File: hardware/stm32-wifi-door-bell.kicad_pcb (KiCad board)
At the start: 2 copper layers, 94 parts, among them J101 USB, M101 Mounting Hole, M102 Mounting Hole, M103 Mounting Hole, M104 Mounting Hole, P101 SWD, P102 FTDI-PLUG, P201 FRONT, P202 BACK, P401 P03, P601 SPEAKER, U101 STM32F072CBT6, U201 OPAMP-DUAL, U202 OPAMP-DUAL, U203 OPAMP-DUAL, U301 MC34063A, U401 TICC3000, U501 MICROSD-AMPHENOL-114-00841-68, U601 LM1875, X101 32.768kHz, X102 8MHz, X401 2500AT44M0400E

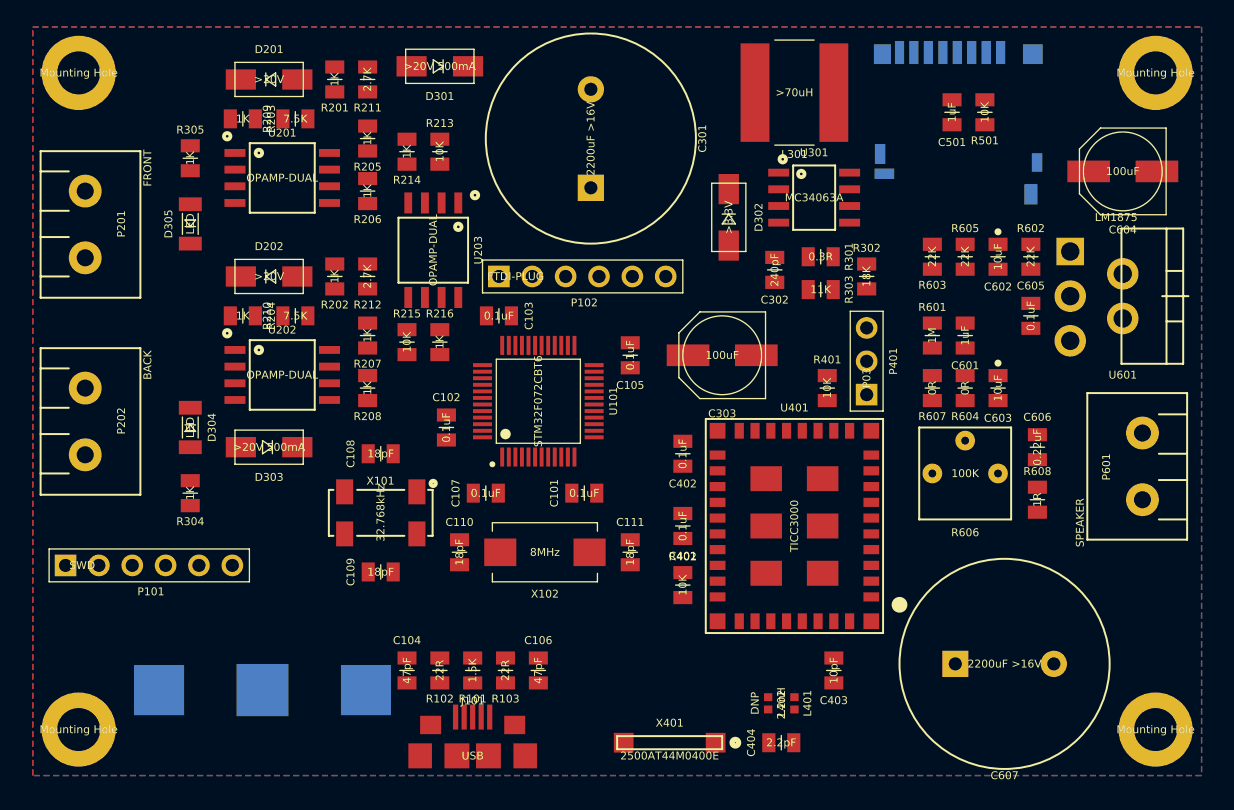
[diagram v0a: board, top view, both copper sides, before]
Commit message: clean up pcb
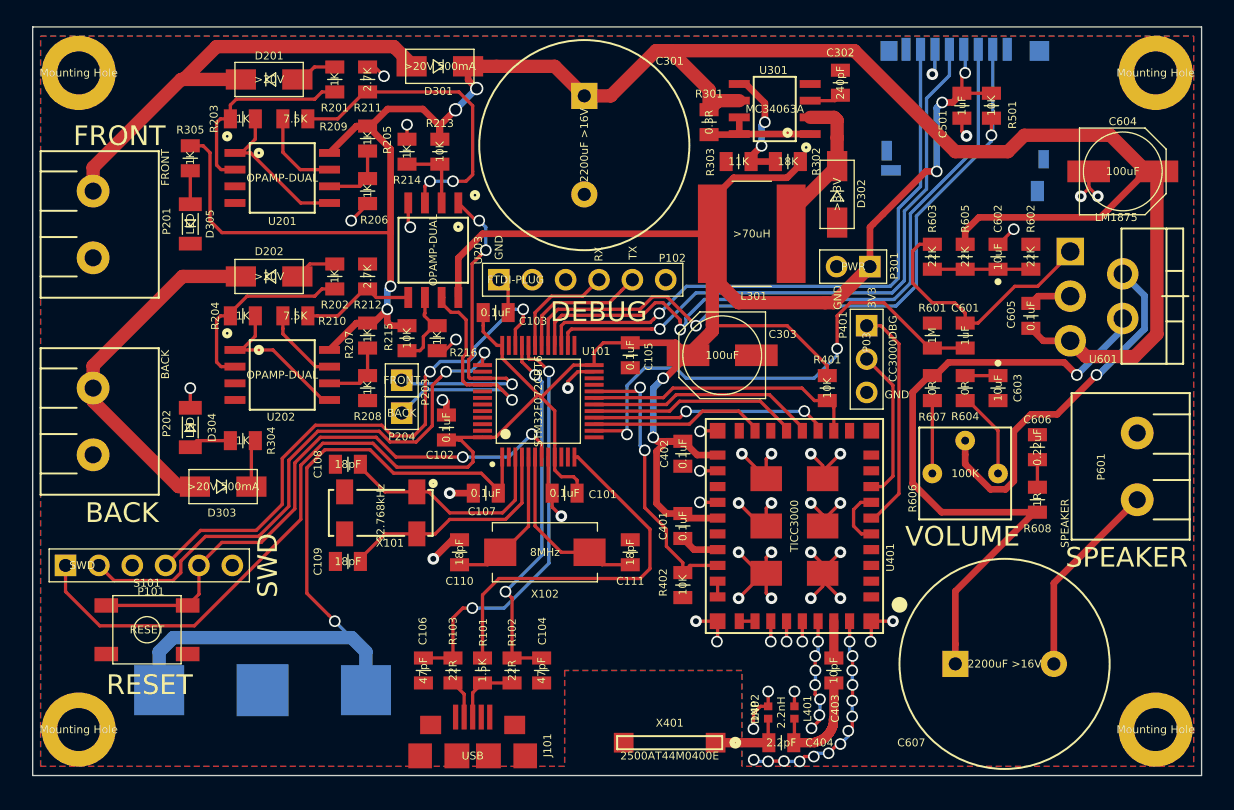
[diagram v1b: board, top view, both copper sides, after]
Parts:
- added P203: FRONT, kicadlib:HDRV1W66P254_1X1_254X249X838P, F.Cu at (88.1, 78.4)
- added P204: BACK, kicadlib:HDRV1W66P254_1X1_254X249X838P, F.Cu at (88.1, 80.9)
- added P301: PWR, kicadlib:HDRV2W66P254_1X2_508X249X838P, F.Cu at (123.8, 69.8)
- added S101: RESET, kicadlib:CKCOMP-PTS525SM10SMTR, F.Cu at (68.7, 97.4)
- P201, P202, P601: footprint kicadlib:OST-OSTTC022162 -> kicadlib:OST-OSTTA024163
- moved C302 15.1 mm to (121.5, 55.8), turned to 90 degrees
- moved R301 13.3 mm to (111.5, 58.8), turned to 270 degrees
- moved R303 11.6 mm to (113.8, 61.8)
- moved L301 11.2 mm to (114.8, 67.2), turned to 180 degrees
- moved R302 10.6 mm to (117.5, 61.8), turned to 0 degrees
- moved C104 10.2 mm to (98.8, 100.5)
- moved C106 8.75 mm to (89.8, 100.5)
- moved D302 8.43 mm to (121.2, 64.2)
- moved U301 7.39 mm to (116.5, 57.8), turned to 180 degrees
- moved R304 5.66 mm to (76.0, 83.0), turned to 0 degrees
- moved R102 5.50 mm to (96.5, 100.5)
- moved P401 5.25 mm to (123.5, 74.2), turned to 270 degrees
- moved D303 4.61 mm to (74.5, 86.5)
- moved R103 4.00 mm to (92.0, 100.5)
- moved C108 2.62 mm to (84.0, 84.8)
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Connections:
- net Net-(C403-Pad1) renamed /wifi/ANT-NET-0
- net Net-(C403-Pad2) renamed /wifi/ANT-NET-1
- net Net-(C404-Pad2) renamed /wifi/ANT-NET-2
- U101 pad 12: Net-(U101-Pad12) -> /USBDPPU
- U101 pad 18: /wifi/CS -> /wifi/IRQ
- U101 pad 19: /wifi/IRQ -> /wifi/CS
- U101 pad 38: /USBDPPU -> Net-(U101-Pad38)
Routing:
- net +3.3V: track 0.00 -> 206.4 mm, vias 0 -> 5
- net Vcc: track 0.00 -> 170.6 mm, vias 0 -> 4
- net GNDPWR: track 0.00 -> 125.1 mm, vias 0 -> 66
- net Net-(BT101-Pad1): track 0.00 -> 56.4 mm, vias 0 -> 1
- net /sdcard/CS: track 0.00 -> 54.6 mm, vias 0 -> 2
- net /sdcard/SPIMOSI: track 0.00 -> 52.4 mm, vias 0 -> 1
- net Net-(C607-Pad1): track 0.00 -> 51.2 mm, vias 0 -> 1
- net /sdcard/CLK: track 0.00 -> 47.3 mm, vias 0 -> 1
- net /sdcard/SPIMISO: track 0.00 -> 46.8 mm, vias 0 -> 1
- net /nRST: track 0.00 -> 44.4 mm, vias 0 -> 2
- net /SWDIO: track 0.00 -> 43.5 mm, vias 0 -> 2
- net /SWCLK: track 0.00 -> 43.3 mm, vias 0 -> 2
- net /audio/AUDIOIN: track 0.00 -> 38.5 mm, vias 0 -> 2
- net /input/FRONTIN: track 0.00 -> 34.9 mm
- net Net-(C106-Pad2): track 0.00 -> 31.9 mm, vias 0 -> 2
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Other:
- board outline added: 89 x 57 mm
- net class ANT added: clearance 0.254, trace_width 0.7112, via_dia 0.889, via_drill 0.635
- net class Default: clearance 0.254 -> 0.2032
- net class POWER added: clearance 0.508, trace_width 1.016, via_dia 1.27, via_drill 1.016
- rule trace_clearance: 0.254 -> 0.2032
- rule trace_min: 0.254 -> 0.1524
- board text added: "3V3"
- board text added: "BACK"
- board text added: "CC3000DBG"
- board text added: "DEBUG"
- board text added: "FRONT"
- board text added: "GND"
- board text added: "RESET"
- board text added: "RX"
- board text added: "SPEAKER"
- board text added: "SWD"
- board text added: "TX"
- board text added: "VOLUME"

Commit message: v20150125
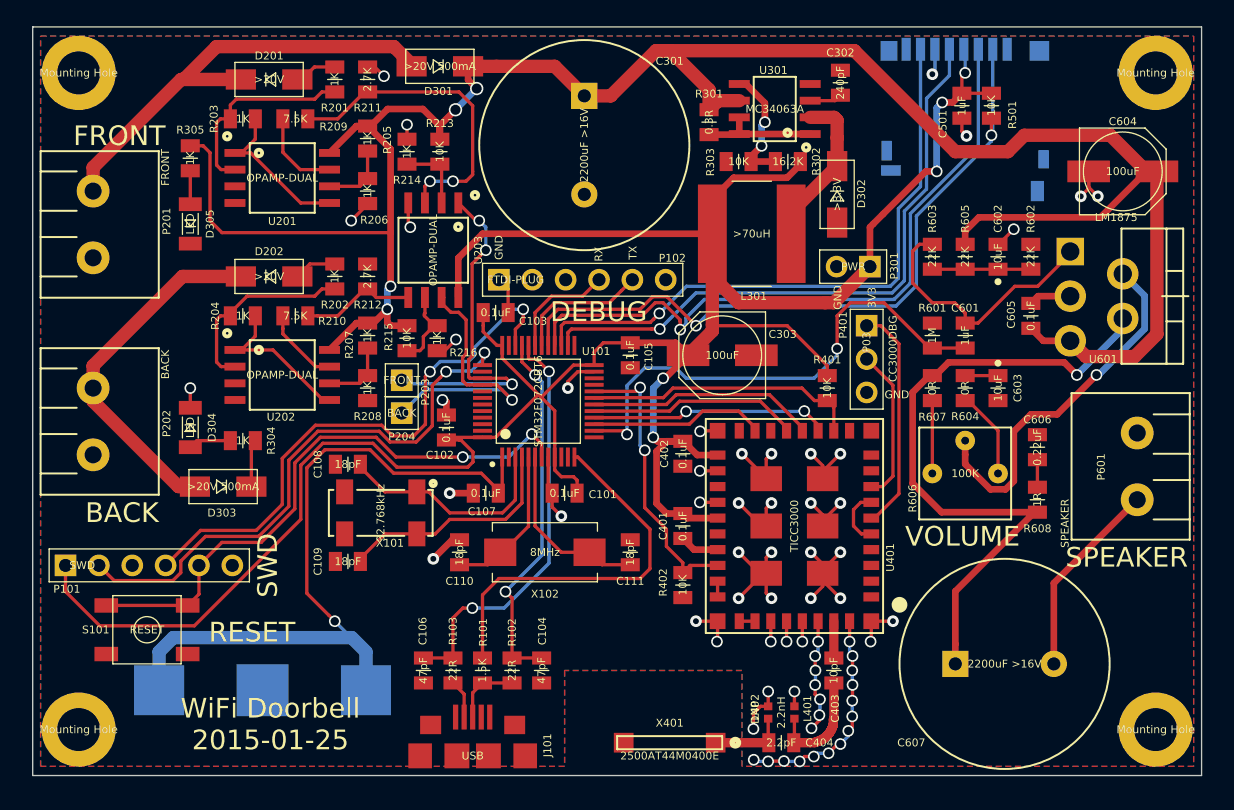
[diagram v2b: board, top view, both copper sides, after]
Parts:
- R302: value 18K -> 16.2K
- R303: value 11K -> 10K
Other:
- board text added: "WiFi Doorbell 2015-01-25"
